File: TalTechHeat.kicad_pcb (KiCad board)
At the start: 4 copper layers, 100 x 30 mm, 77 parts, among them J1 02x03, J2 OLED_SSD1306, J3 XT-30, J4 Conn_01x04, Q1 DMP4015SPSQ-13, Q2 PJQ4439EP-AU_R2_002A1, Q3 PJQ4439EP-AU_R2_002A1, Q4 IRLR8726TRPBF, Q5 SS8050-G, SW1 Reset_Switch, SW2 BUT1, SW3 BUT2, U1 STM32F103C6Tx, U2 AP64060ZQ, U3 USB-C, U4 STUSB4500, Y1 8 MHz

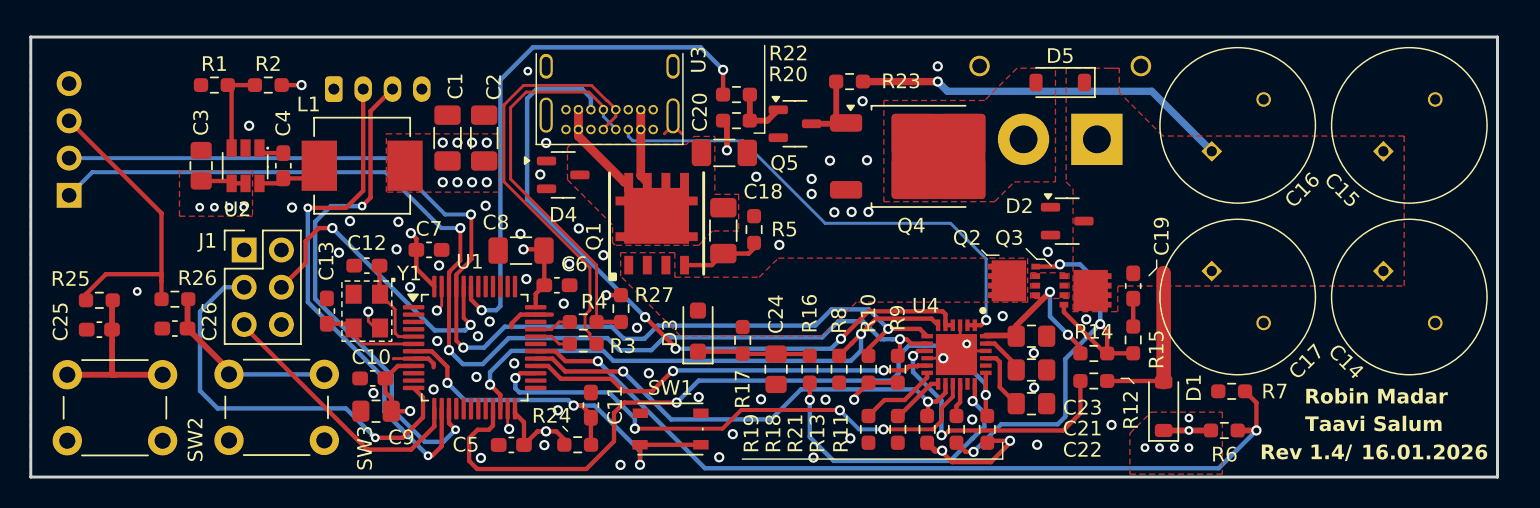
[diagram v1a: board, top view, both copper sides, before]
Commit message: Fixes implementation 1/2
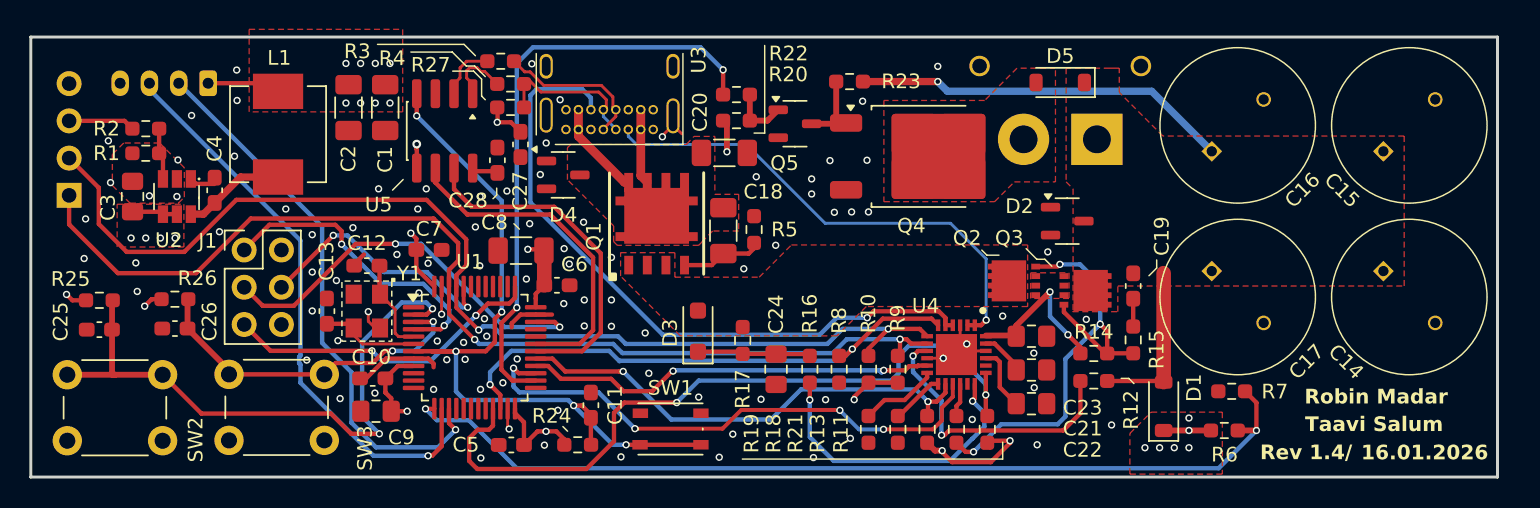
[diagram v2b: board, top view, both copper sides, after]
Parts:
- added C27: 100nF, Capacitor_SMD:C_0603_1608Metric_Pad1.08x0.95mm_HandSolder, F.Cu at (184.8, 93.0)
- added C28: 100nF, Capacitor_SMD:C_0603_1608Metric_Pad1.08x0.95mm_HandSolder, F.Cu at (183.3, 94.1)
- added U5: ~, Package_SO:SOP-8_3.76x4.96mm_P1.27mm, F.Cu at (179.7, 92.1)
- moved R3 20.1 mm to (183.5, 87.3)
- moved R4 17.0 mm to (184.2, 88.9)
- moved R27 15.6 mm to (184.2, 90.5), turned to 180 degrees
- moved C2 9.48 mm to (173.1, 90.5), turned to -90 degrees
- moved R2 8.87 mm to (159.3, 91.9), turned to 180 degrees
- moved J4 8.58 mm to (163.6, 88.8), turned to 180 degrees
- moved R1 6.60 mm to (159.3, 93.6)
- moved G*** 6.37 mm to (168.1, 94.9)
- moved L1 6.12 mm to (168.3, 92.3), turned to 90 degrees
- moved C3 5.13 mm to (158.4, 96.5)
- moved U2 5.13 mm to (161.4, 96.5)
- moved C4 4.97 mm to (164.0, 96.1)
- moved C1 4.73 mm to (175.6, 90.5), turned to -90 degrees
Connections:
- J1 pad 1: unconnected-(J1-Pin_1-Pad1) -> /PC15
- J1 pad 3: /UART2_TX -> /SWDIO
- J1 pad 5: /UART2_RX -> /SWCLK
- J4 pad 2: /TEMP_1 -> /TEMP_2
- J4 pad 3: /TEMP_2 -> /TEMP_1
- U1 pad 12: /UART2_TX -> unconnected-(U1-PA2-Pad12)
- U1 pad 13: /UART2_RX -> /VCC-DIV
- U1 pad 2: unconnected-(U1-PC13-Pad2) -> /BUT1
- U1 pad 26: unconnected-(U1-PB13-Pad26) -> /PWM
- U1 pad 3: unconnected-(U1-PC14-Pad3) -> /BUT2
- U1 pad 30: /VCC-DIV -> /UART1_RX
- U1 pad 31: unconnected-(U1-PA10-Pad31) -> /UART1_TX
- U1 pad 32: /D_N -> unconnected-(U1-PA11-Pad32)
- U1 pad 33: /D_P -> unconnected-(U1-PA12-Pad33)
- U1 pad 34: unconnected-(U1-PA13-Pad34) -> /SWDIO
- U1 pad 37: unconnected-(U1-PA14-Pad37) -> /SWCLK
- U1 pad 4: unconnected-(U1-PC15-Pad4) -> /PC15
- U1 pad 43: /PWM -> unconnected-(U1-PB7-Pad43)
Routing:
- net /BUT1: track 11.8 -> 42.5 mm, vias 0 -> 2
- net /UART2_TX: track 28.5 -> 0.00 mm, vias 1 -> 0
- net /SWDIO: track 0.00 -> 27.9 mm, vias 0 -> 2
- net /UART1_RX: track 0.00 -> 23.6 mm
- net /UART1_TX: track 0.00 -> 23.1 mm
- net /NRST: track 28.8 -> 51.4 mm, vias 3 -> 5
- net /SWCLK: track 0.00 -> 22.1 mm, vias 0 -> 2
- net /PC15: track 0.00 -> 21.0 mm, vias 0 -> 2
- net /U_N: track 29.8 -> 10.4 mm
- net /UART2_RX: track 18.4 -> 0.00 mm
- net /U_P: track 27.8 -> 10.3 mm
- net /BUT2: track 12.8 -> 23.5 mm, vias 0 -> 2
- net +3.3V: track 60.4 -> 53.9 mm, vias 18 -> 20
- net /VCC-DIV: track 57.8 -> 64.3 mm
- net /TEMP_1: track 35.2 -> 39.3 mm, vias 2 -> 1
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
